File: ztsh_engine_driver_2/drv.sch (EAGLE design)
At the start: 57 parts, among them IC1 74AC14N, Q1 IRF640N, Q2 IRF640N, Q3 IRF640N, Q4 IRF640N, U1 IR2110-1PBF, U2 IR2110-1PBF

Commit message: board update
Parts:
- Q1, Q2, Q3, Q4: device transistor-power:IRF3704 -> transistor-power:IRF3704L-V
- R11, R12: device rcl:R-EU_R0805 -> rcl:R-EU_0204/2V
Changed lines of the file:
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@@
 <grid distance="0.1" unitdist="inch" unit="inch" style="lines" multiple="1" display="no" altdistance="0.01" altunitdist="inch" altunit="inch"/>
 <layers>
-<layer number="1" name="Top" color="4" fill="1" visible="no" active="no"/>
-<layer number="2" name="Route2" color="1" fill="3" visible="no" active="no"/>
-<layer number="3" name="Route3" color="4" fill="3" visible="no" active="no"/>
-<layer number="4" name="Route4" color="1" fill="4" visible="no" active="no"/>
-<layer number="5" name="Route5" color="4" fill="4" visible="no" active="no"/>
-<layer number="6" name="Route6" color="1" fill="8" visible="no" active="no"/>
-<layer number="7" name="Route7" color="4" fill="8" visible="no" active="no"/>
-<layer number="8" name="Route8" color="1" fill="2" visible="no" active="no"/>
-<layer number="9" name="Route9" color="4" fill="2" visible="no" active="no"/>
-<layer number="10" name="Route10" color="1" fill="7" visible="no" active="no"/>
-<layer number="11" name="Route11" color="4" fill="7" visible="no" active="no"/>
-<layer number="12" name="Route12" color="1" fill="5" visible="no" active="no"/>
-<layer number="13" name="Route13" color="4" fill="5" visible="no" active="no"/>
-<layer number="14" name="Route14" color="1" fill="6" visible="no" active="no"/>
-<layer number="15" name="Route15" color="4" fill="6" visible="no" active="no"/>
-<layer number="16" name="Bottom" color="1" fill="1" visible="no" active="no"/>
-<layer number="17" name="Pads" color="2" fill="1" visible="no" active="no"/>
-<layer number="18" name="Vias" color="2" fill="1" visible="no" active="no"/>
-<layer number="19" name="Unrouted" color="6" fill="1" visible="no" active="no"/>
-<layer number="20" name="Dimension" color="15" fill="1" visible="no" active="no"/>
-<layer number="21" name="tPlace" color="7" fill="1" visible="no" active="no"/>
-<layer number="22" name="bPlace" color="7" fill="1" visible="no" active="no"/>
-<layer number="23" name="tOrigins" color="15" fill="1" visible="no" active="no"/>
-<layer number="24" name="bOrigins" color="15" fill="1" visible="no" active="no"/>
-<layer number="25" name="tNames" color="7" fill="1" visible="no" active="no"/>
-<layer number="26" name="bNames" color="7" fill="1" visible="no" active="no"/>
-<layer number="27" name="tValues" color="7" fill="1" visible="no" active="no"/>
-<layer number="28" name="bValues" color="7" fill="1" visible="no" active="no"/>
+<layer number="1" name="Top" color="4" fill="1" visible="yes" active="no"/>
+<layer number="2" name="Route2" color="1" fill="3" visible="yes" active="no"/>
+<layer number="3" name="Route3" color="4" fill="3" visible="yes" active="no"/>
+<layer number="4" name="Route4" color="1" fill="4" visible="yes" active="no"/>
+<layer number="5" name="Route5" color="4" fill="4" visible="yes" active="no"/>
+<layer number="6" name="Route6" color="1" fill="8" visible="yes" active="no"/>
+<layer number="7" name="Route7" color="4" fill="8" visible="yes" active="no"/>
+<layer number="8" name="Route8" color="1" fill="2" visible="yes" active="no"/>
+<layer number="9" name="Route9" color="4" fill="2" visible="yes" active="no"/>
+<layer number="10" name="Route10" color="1" fill="7" visible="yes" active="no"/>
+<layer number="11" name="Route11" color="4" fill="7" visible="yes" active="no"/>
+<layer number="12" name="Route12" color="1" fill="5" visible="yes" active="no"/>
+<layer number="13" name="Route13" color="4" fill="5" visible="yes" active="no"/>
+<layer number="14" name="Route14" color="1" fill="6" visible="yes" active="no"/>
+<layer number="15" name="Route15" color="4" fill="6" visible="yes" active="no"/>
+<layer number="16" name="Bottom" color="1" fill="1" visible="yes" active="no"/>
+<layer number="17" name="Pads" color="2" fill="1" visible="yes" active="no"/>
+<layer number="18" name="Vias" color="2" fill="1" visible="yes" active="no"/>
+<layer number="19" name="Unrouted" color="6" fill="1" visible="yes" active="no"/>
+<layer number="20" name="Dimension" color="15" fill="1" visible="yes" active="no"/>
+<layer number="21" name="tPlace" color="7" fill="1" visible="yes" active="no"/>
+<layer number="22" name="bPlace" color="7" fill="1" visible="yes" active="no"/>
+<layer number="23" name="tOrigins" color="15" fill="1" visible="yes" active="no"/>
+<layer number="24" name="bOrigins" color="15" fill="1" visible="yes" active="no"/>
+<layer number="25" name="tNames" color="7" fill="1" visible="yes" active="no"/>
+<layer number="26" name="bNames" color="7" fill="1" visible="yes" active="no"/>
+<layer number="27" name="tValues" color="7" fill="1" visible="yes" active="no"/>
+<layer number="28" name="bValues" color="7" fill="1" visible="yes" active="no"/>
 <layer number="29" name="tStop" color="7" fill="3" visible="no" active="no"/>
 <layer number="30" name="bStop" color="7" fill="6" visible="no" active="no"/>
@@
 <layer number="35" name="tGlue" color="7" fill="4" visible="no" active="no"/>
 <layer number="36" name="bGlue" color="7" fill="5" visible="no" active="no"/>
-<layer number="37" name="tTest" color="7" fill="1" visible="no" active="no"/>
-<layer number="38" name="bTest" color="7" fill="1" visible="no" active="no"/>
+<layer number="37" name="tTest" color="7" fill="1" visible="yes" active="no"/>
+<layer number="38" name="bTest" color="7" fill="1" visible="yes" active="no"/>
 <layer number="39" name="tKeepout" color="4" fill="11" visible="no" active="no"/>
 <layer number="40" name="bKeepout" color="1" fill="11" visible="no" active="no"/>
@@
 <layer number="44" name="Drills" color="7" fill="1" visible="no" active="no"/>
 <layer number="45" name="Holes" color="7" fill="1" visible="no" active="no"/>
-<layer number="46" name="Milling" color="3" fill="1" visible="no" active="no"/>
-<layer number="47" name="Measures" color="7" fill="1" visible="no" active="no"/>
-<layer number="48" name="Document" color="7" fill="1" visible="no" active="no"/>
-<layer number="49" name="Reference" color="7" fill="1" visible="no" active="no"/>
-<layer number="50" name="dxf" color="7" fill="1" visible="no" active="no"/>
-<layer number="51" name="tDocu" color="7" fill="1" visible="no" active="no"/>
-<layer number="52" name="bDocu" color="7" fill="1" visible="no" active="no"/>
-<layer number="53" name="tGND_GNDA" color="7" fill="9" visible="no" active="no"/>
-<layer number="54" name="bGND_GNDA" color="1" fill="9" visible="no" active="no"/>
-<layer number="56" name="wert" color="7" fill="1" visible="no" active="no"/>
-<layer number="57" name="tCAD" color="7" fill="1" visible="no" active="no"/>
+<layer number="46" name="Milling" color="3" fill="1" visible="yes" active="no"/>
+<layer number="47" name="Measures" color="7" fill="1" visible="yes" active="no"/>
+<layer number="48" name="Document" color="7" fill="1" visible="yes" active="no"/>
+<layer number="49" name="Reference" color="7" fill="1" visible="yes" active="no"/>
+<layer number="50" name="dxf" color="7" fill="1" visible="yes" active="no"/>
+<layer number="51" name="tDocu" color="7" fill="1" visible="yes" active="no"/>
+<layer number="52" name="bDocu" color="7" fill="1" visible="yes" active="no"/>
+<layer number="53" name="tGND_GNDA" color="7" fill="9" visible="yes" active="no"/>
+<layer number="54" name="bGND_GNDA" color="1" fill="9" visible="yes" active="no"/>
+<layer number="56" name="wert" color="7" fill="1" visible="yes" active="no"/>
+<layer number="57" name="tCAD" color="7" fill="1" visible="yes" active="no"/>
 <layer number="90" name="Modules" color="5" fill="1" visible="yes" active="yes"/>
 <layer number="91" name="Nets" color="2" fill="1" visible="yes" active="yes"/>
@@
 </classes>
 <parts>
-<part name="Q1" library="transistor-power" deviceset="IRF3704" device="" value="IRF640N"/>
-<part name="Q2" library="transistor-power" deviceset="IRF3704" device="" value="IRF640N"/>
-<part name="Q3" library="transistor-power" deviceset="IRF3704" device="" value="IRF640N"/>
-<part name="Q4" library="transistor-power" deviceset="IRF3704" device="" value="IRF640N"/>
+<part name="Q1" library="transistor-power" deviceset="IRF3704" device="L-V" value="IRF640N"/>
+<part name="Q2" library="transistor-power" deviceset="IRF3704" device="L-V" value="IRF640N"/>
+<part name="Q3" library="transistor-power" deviceset="IRF3704" device="L-V" value="IRF640N"/>
+<part name="Q4" library="transistor-power" deviceset="IRF3704" device="L-V" value="IRF640N"/>
 <part name="U1" library="International_Rectifier_By_element14_Batch_1" deviceset="IR2110-1PBF" device=""/>
 <part name="U2" library="International_Rectifier_By_element14_Batch_1" deviceset="IR2110-1PBF" device=""/>
@@
 <part name="GND5" library="SparkFun-Aesthetics" deviceset="GND" device=""/>
 <part name="GND6" library="SparkFun-Aesthetics" deviceset="GND" device=""/>
-<part name="R11" library="rcl" deviceset="R-EU_" device="R0805"/>
-<part name="R12" library="rcl" deviceset="R-EU_" device="R0805"/>
+<part name="R11" library="rcl" deviceset="R-EU_" device="0204/2V"/>
+<part name="R12" library="rcl" deviceset="R-EU_" device="0204/2V"/>
 <part name="GND13" library="SparkFun-Aesthetics" deviceset="GND" device=""/>
 <part name="GND14" library="SparkFun-Aesthetics" deviceset="GND" device=""/>

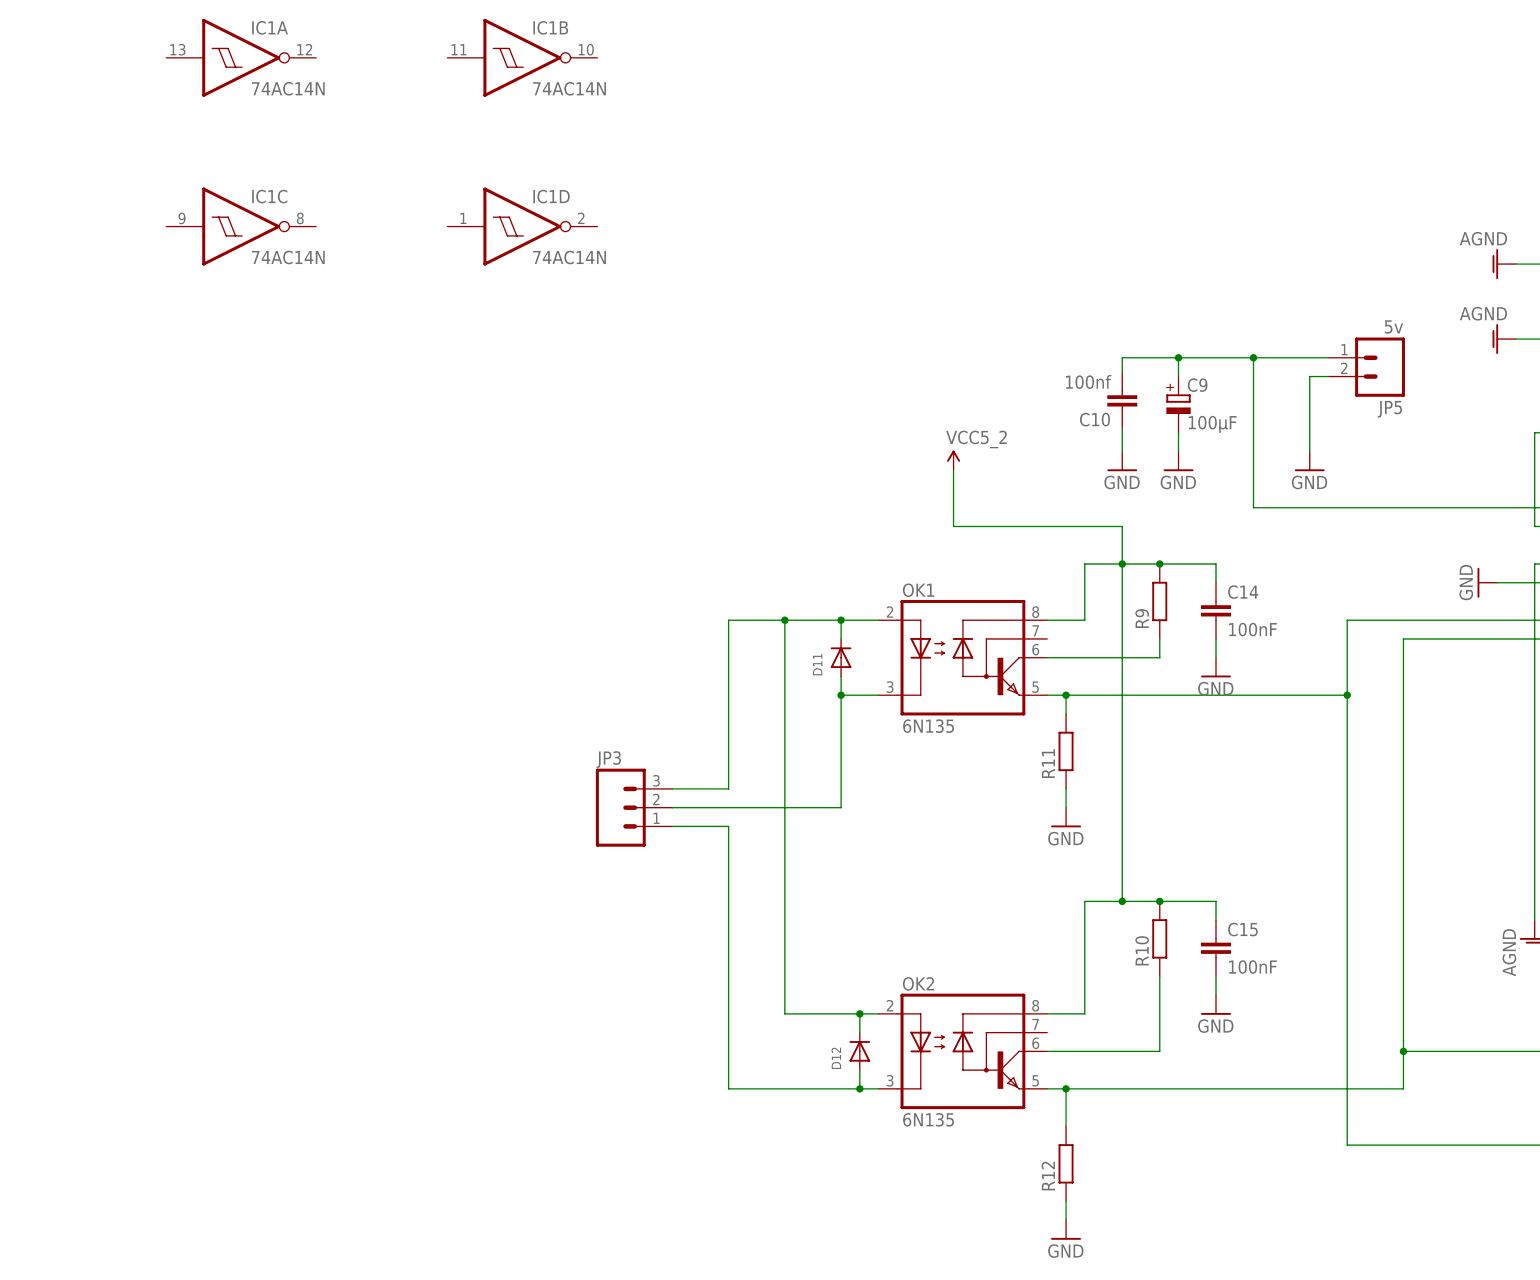
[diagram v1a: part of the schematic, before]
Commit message: board update (near finish, hope...)
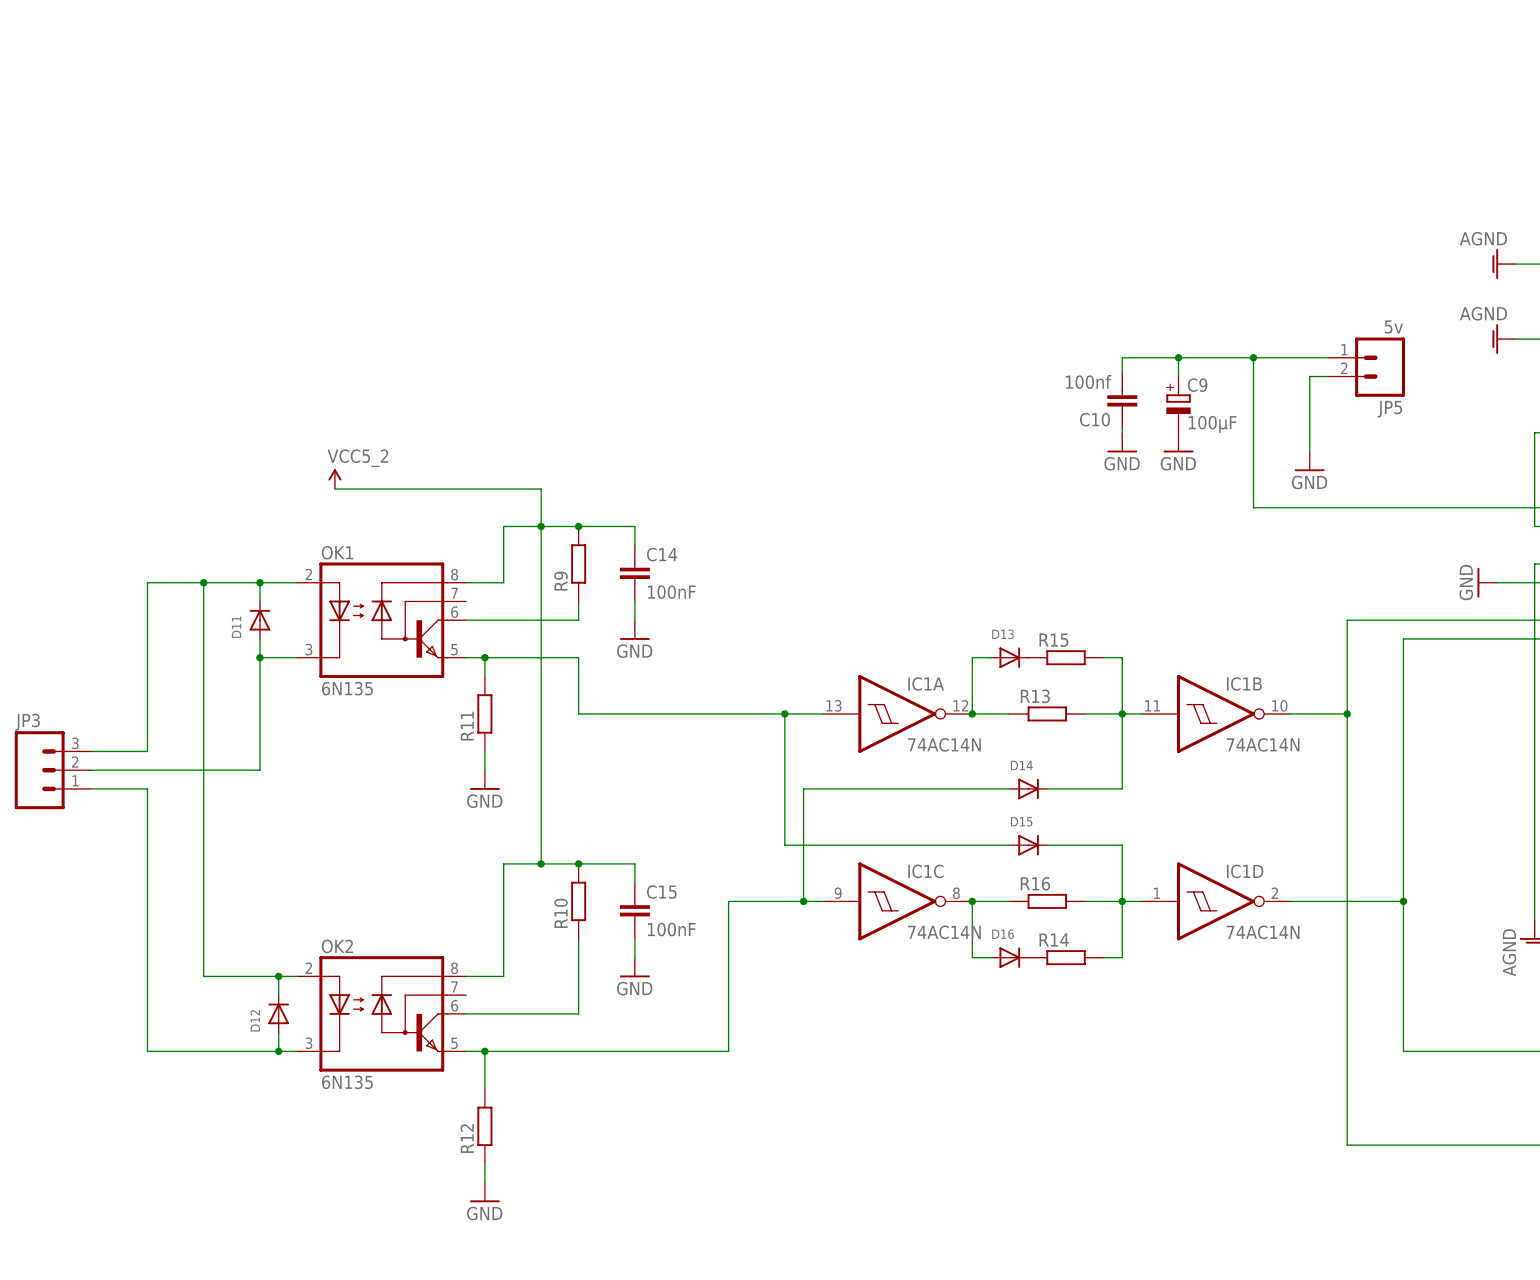
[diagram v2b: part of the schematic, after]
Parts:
- added D13, D14, D15, D16: (no value), adafruit:DIODEDO-1N4148
- added R13, R14, R15, R16: (no value), resistor:R-EU_0204/7
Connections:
- new net N$18: D14.A, IC1C.I, OK2.GND, R12.2
- new net N$2: D15.A, IC1A.I, OK1.GND, R11.2
- new net N$20: D13.C, R15.1
- new net N$21: D14.C, IC1B.I, R13.2, R15.2
- new net N$22: D13.A, IC1A.O, R13.1
- new net N$23: D16.C, R14.1
- new net N$24: D15.C, IC1D.I, R14.2, R16.2
- new net N$25: D16.A, IC1C.O, R16.1
- net N$16: now also IC1B.O; no longer OK1.GND, R11.2
- net N$19: now also IC1D.O; no longer OK2.GND, R12.2
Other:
- moved on the sheet: C14, C15, D11, D12, IC1A, IC1B, IC1C, IC1D, JP3, OK1, OK2, R10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
